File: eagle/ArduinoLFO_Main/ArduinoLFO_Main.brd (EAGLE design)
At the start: 70.8 x 45.7 mm, 23 parts, among them IC1 MCP4922

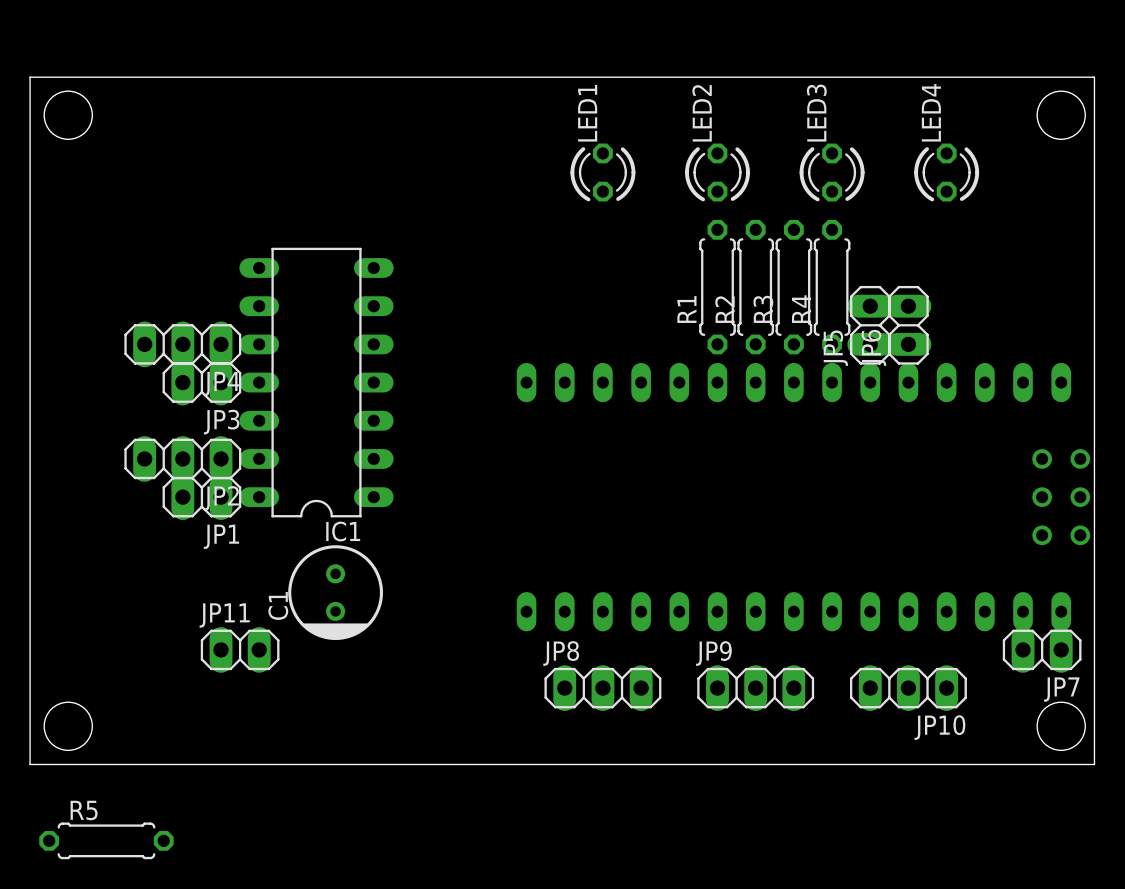
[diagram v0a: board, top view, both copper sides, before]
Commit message: Board Design
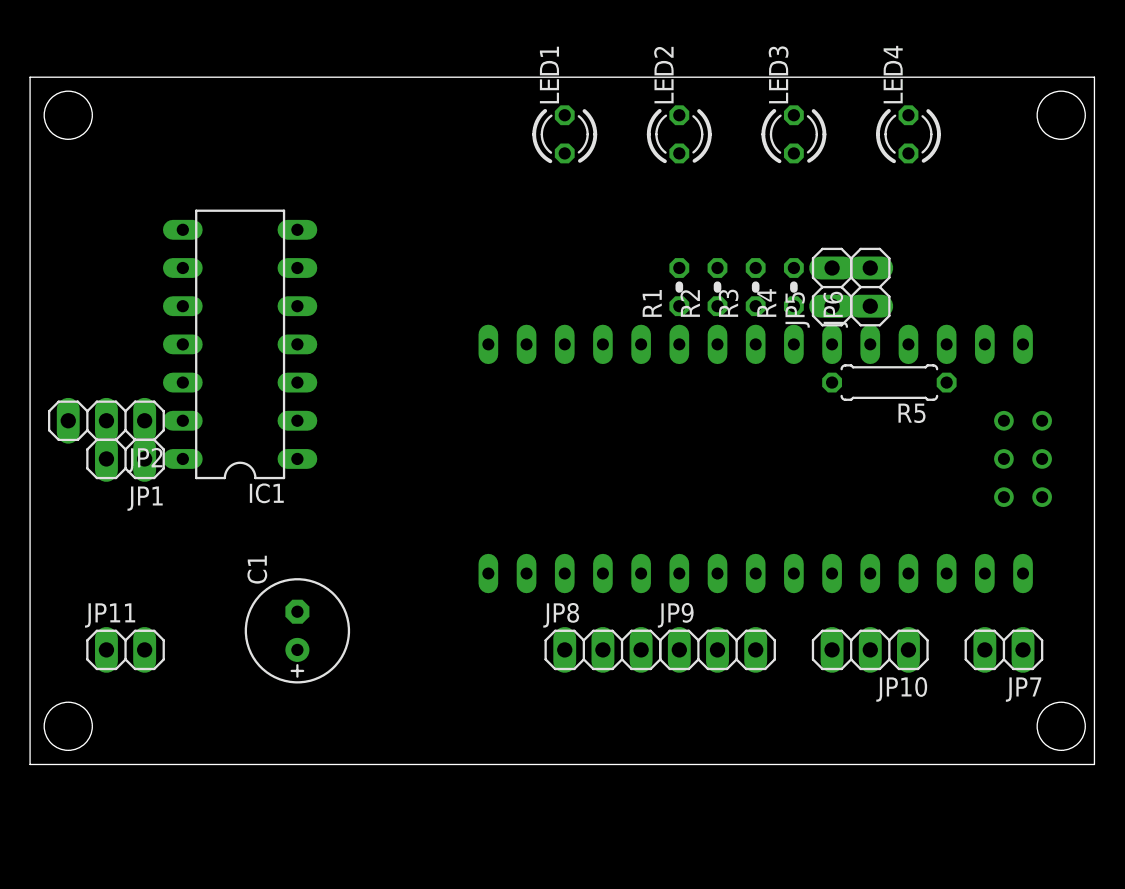
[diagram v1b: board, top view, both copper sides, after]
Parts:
- removed JP3: OUTB, pinhead:1X02
- removed JP4: VREFB, pinhead:1X03
- C1: device rcl:SANYO-OSCON_C6 -> rcl:E2,5-7
- R1, R2, R3, R4: device rcl:0207/7 -> rcl:0204V
- moved R5 60.3 mm to (57.1, 25.4), turned to 180 degrees
- moved JP11 7.62 mm to (6.35, 7.62)
- moved IC1 5.68 mm to (14.0, 26.7)
- moved JP1 5.68 mm to (6.35, 20.3)
- moved JP2 5.68 mm to (5.08, 22.9)
- moved LED3 3.59 mm to (50.8, 41.9)
- moved JP10 3.59 mm to (55.9, 7.62)
- moved JP9 3.59 mm to (45.7, 7.62)
- moved C1 3.59 mm to (17.8, 8.89)
- moved JP5 3.59 mm to (53.3, 31.8)
- moved JP6 3.59 mm to (55.9, 31.8)
- moved LED1 3.59 mm to (35.6, 41.9)
- moved LED2 3.59 mm to (43.2, 41.9)
- moved LED4 3.59 mm to (58.4, 41.9)
- moved U$1 3.59 mm to (57.1, 22.9)
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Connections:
- removed net N$4: IC1.8, U$1.D9
- removed net N$8: IC1.11, JP3.1
- removed net N$9: IC1.10, JP4.1
- net +3V3: no longer JP4.3
- net GND: now also IC1.11; no longer JP3.2, JP4.2
